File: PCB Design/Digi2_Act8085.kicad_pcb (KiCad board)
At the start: 2 copper layers, 27 parts, among them U1 8085A, U10 8255, U2 Barrel_Jack, U3 L7805, U4 2764, U5 CY6264, U6 74LS373, U7 74LS138, U8 8255, U9 8255, Y1 3MHz

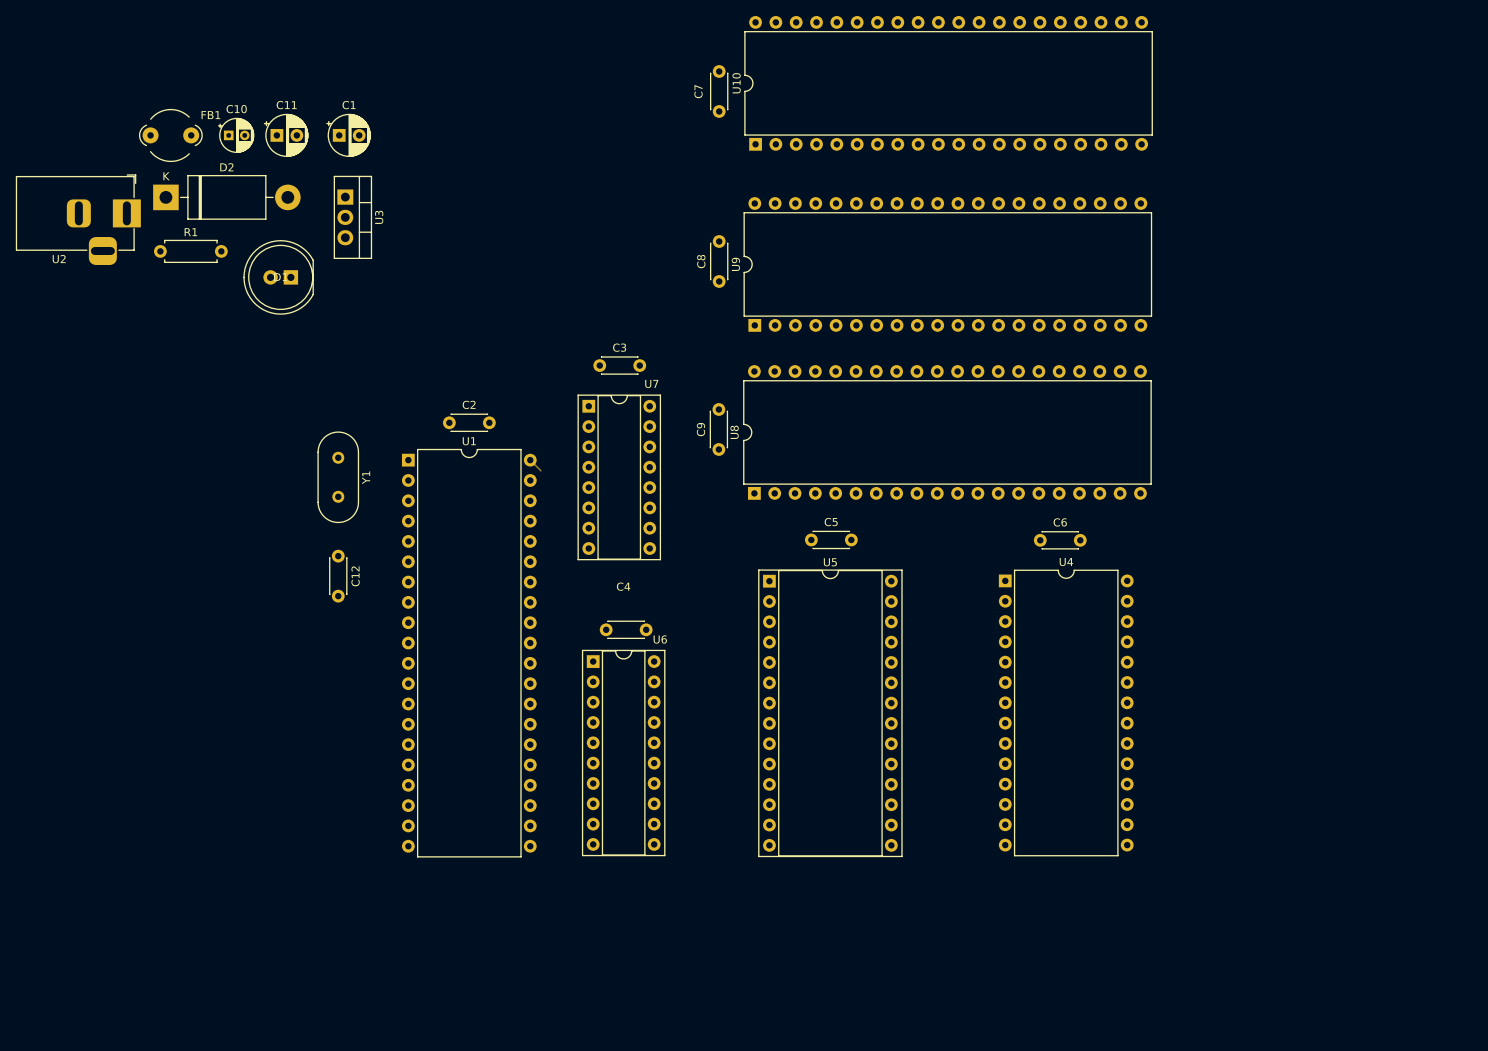
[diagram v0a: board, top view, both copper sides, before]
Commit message: Initial B
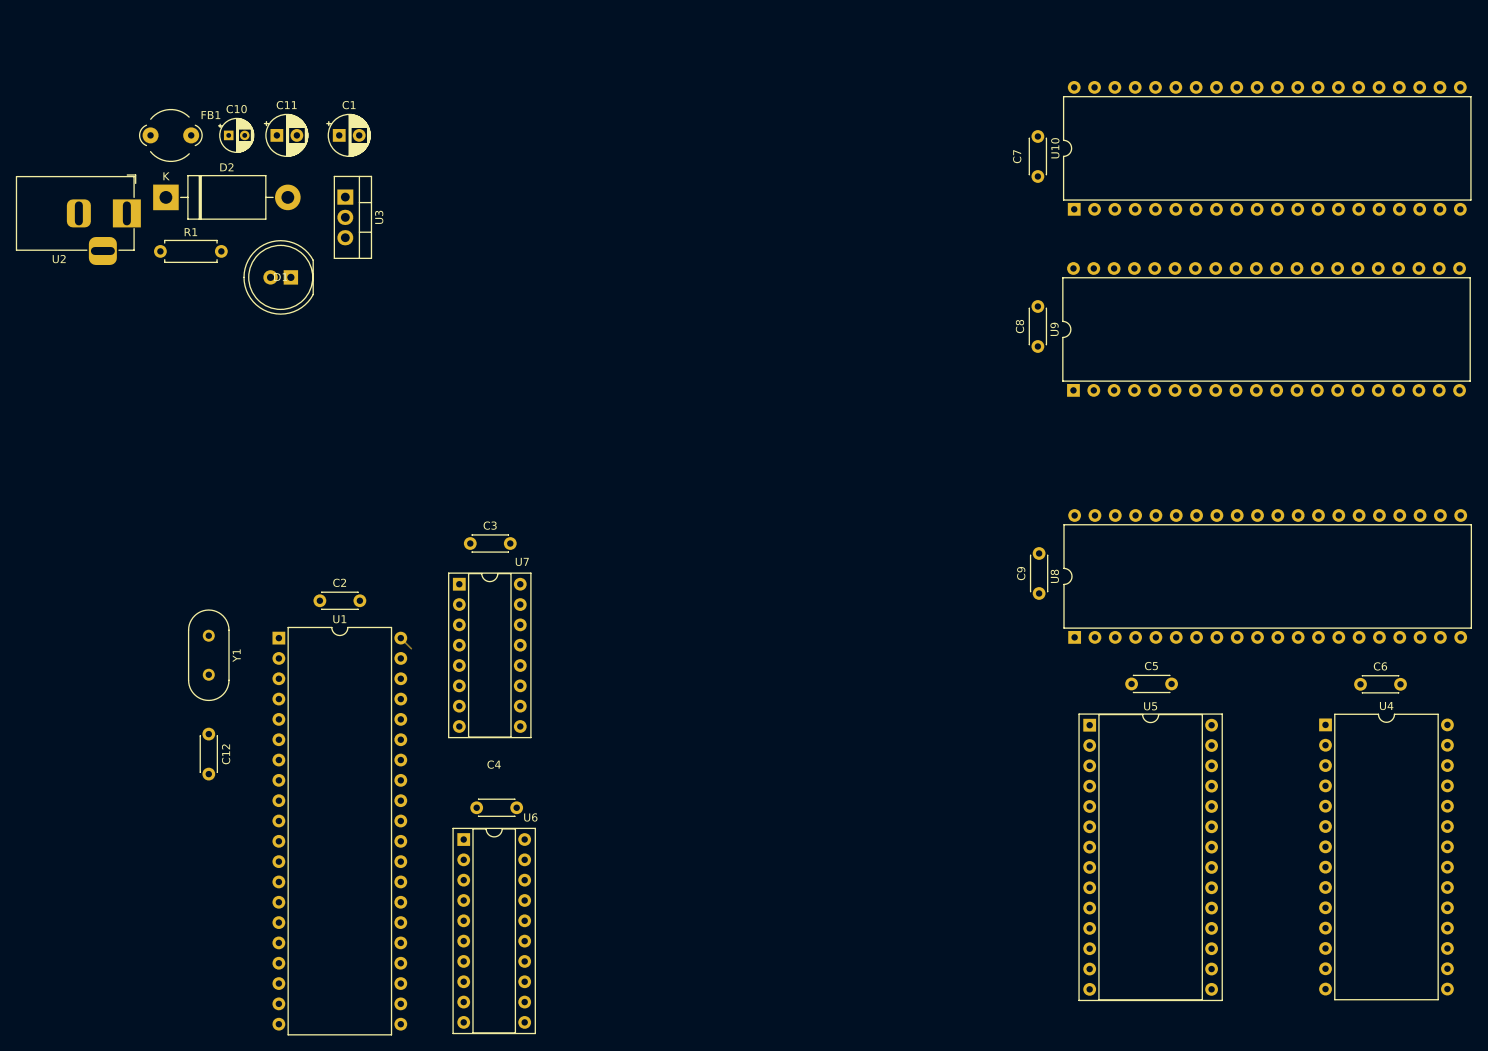
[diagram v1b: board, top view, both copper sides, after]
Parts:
- moved C5 43.9 mm to (168.1, 116.1)
- moved C6 43.9 mm to (196.7, 116.1)
- moved C9 43.9 mm to (156.5, 104.8)
- moved U4 43.9 mm to (192.3, 121.2)
- moved U5 43.9 mm to (162.8, 121.2)
- moved U8 43.9 mm to (161.0, 110.2)
- moved C7 40.7 mm to (156.4, 52.6)
- moved C8 40.7 mm to (156.4, 73.9)
- moved U10 40.7 mm to (160.9, 56.7)
- moved U9 40.7 mm to (160.8, 79.4)
- moved C2 27.5 mm to (66.6, 105.7)
- moved C3 27.5 mm to (85.4, 98.5)
- moved U1 27.5 mm to (61.5, 110.3)
- moved C12 27.5 mm to (52.7, 122.3)
- moved U7 27.5 mm to (84.1, 103.6)
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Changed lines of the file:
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@@
 	(footprint "Capacitor_THT:C_Disc_D4.3mm_W1.9mm_P5.00mm"
 		(layer "F.Cu")
-		(at 82.81 83.425)
+		(at 66.625 105.67)
 		(descr "C, Disc series, Radial, pin pitch=5.00mm, , diameter*width=4.3*1.9mm^2, Capacitor, http://www.vishay.com/docs/45233/krseries.pdf")
 		(tags "C Disc series Radial pin pitch 5.00mm  diameter 4.3mm width 1.9mm Capacitor")
@@
 	(footprint "Crystal:Crystal_HC49-U_Vertical"
 		(layer "F.Cu")
-		(at 68.925 87.795 -90)
+		(at 52.74 110.04 -90)
 		(descr "Crystal THT HC-49/U http://5hertz.com/pdfs/04404_D.pdf")
 		(tags "THT crystalHC-49/U")
@@
 	(footprint "Package_DIP:DIP-16_W7.62mm_Socket"
 		(layer "F.Cu")
-		(at 100.24 81.36)
+		(at 84.055 103.605)
 		(descr "16-lead though-hole mounted DIP package, row spacing 7.62 mm (300 mils), Socket")
 		(tags "THT DIP DIL PDIP 2.54mm 7.62mm 300mil Socket")
@@
 	(footprint "Package_DIP:DIP-20_W7.62mm_Socket"
 		(layer "F.Cu")
-		(at 100.79 113.27)
+		(at 84.605 135.515)
 		(descr "20-lead though-hole mounted DIP package, row spacing 7.62 mm (300 mils), Socket")
 		(tags "THT DIP DIL PDIP 2.54mm 7.62mm 300mil Socket")
 		(property "Reference" "U6"
-			(at 8.37 -2.72 360)
+			(at 8.37 -2.72 0)
 			(layer "F.SilkS")
 			(effects
@@
 		)
 		(property "Value" "74LS373"
-			(at 7.945 26.37 360)
+			(at 7.945 26.37 0)
 			(layer "F.Fab")
 			(effects
@@
 		)
 		(fp_text user "${REFERENCE}"
-			(at 7.945 12.61 360)
+			(at 7.945 12.61 0)
 			(layer "F.Fab")
 			(effects
@@
 	(footprint "Capacitor_THT:C_Disc_D4.3mm_W1.9mm_P5.00mm"
 		(layer "F.Cu")
-		(at 116.5 86.76 90)
+		(at 156.53 104.76 90)
 		(descr "C, Disc series, Radial, pin pitch=5.00mm, , diameter*width=4.3*1.9mm^2, Capacitor, http://www.vishay.com/docs/45233/krseries.pdf")
 		(tags "C Disc series Radial pin pitch 5.00mm  diameter 4.3mm width 1.9mm Capacitor")
 		(property "Reference" "C9"
-			(at 2.5 -2.2 270)
+			(at 2.5 -2.2 -90)
 			(layer "F.SilkS")
 			(effects
@@
 		)
 		(property "Value" "100nF"
-			(at 2.5 2.2 270)
+			(at 2.5 2.2 -90)
 			(layer "F.Fab")
 			(effects
@@
 		)
 		(fp_text user "${REFERENCE}"
-			(at 2.5 0 270)
+			(at 2.5 0 -90)
 			(layer "F.Fab")
 			(effects
@@
 	(footprint "Package_DIP:DIP-40_W15.24mm"
 		(layer "F.Cu")
-		(at 121.085 48.615 90)
+		(at 160.92 56.74 90)
 		(descr "40-lead though-hole mounted DIP package, row spacing 15.24 mm (600 mils)")
 		(tags "THT DIP DIL PDIP 2.54mm 15.24mm 600mil")
 		(property "Reference" "U10"
-			(at 7.62 -2.33 270)
+			(at 7.62 -2.33 -90)
 			(layer "F.SilkS")
 			(effects
@@
 		)
 		(property "Value" "8255"
-			(at 7.62 50.59 270)
+			(at 7.62 50.59 -90)
 			(layer "F.Fab")
 			(effects
@@
 		)
 		(fp_text user "${REFERENCE}"
-			(at 7.62 24.13 270)
+			(at 7.62 24.13 -90)
 			(layer "F.Fab")
 			(effects
@@
 	(footprint "Capacitor_THT:C_Disc_D4.3mm_W1.9mm_P5.00mm"
 		(layer "F.Cu")
-		(at 101.61 76.27)
+		(at 85.425 98.515)
 		(descr "C, Disc series, Radial, pin pitch=5.00mm, , diameter*width=4.3*1.9mm^2, Capacitor, http://www.vishay.com/docs/45233/krseries.pdf")
 		(tags "C Disc series Radial pin pitch 5.00mm  diameter 4.3mm width 1.9mm Capacitor")
@@
 	(footprint "Package_DIP:DIP-28_W15.24mm_Socket"
 		(layer "F.Cu")
-		(at 122.82 103.225)
+		(at 162.85 121.225)
 		(descr "28-lead though-hole mounted DIP package, row spacing 15.24 mm (600 mils), Socket")
 		(tags "THT DIP DIL PDIP 2.54mm 15.24mm 600mil Socket")
@@
 	(footprint "Package_DIP:DIP-28_W15.24mm"
 		(layer "F.Cu")
-		(at 152.3 103.19)
+		(at 192.33 121.19)
 		(descr "28-lead though-hole mounted DIP package, row spacing 15.24 mm (600 mils)")
 		(tags "THT DIP DIL PDIP 2.54mm 15.24mm 600mil")
@@
 	(footprint "Capacitor_THT:C_Disc_D4.3mm_W1.9mm_P5.00mm"
 		(layer "F.Cu")
-		(at 116.54 65.76 90)
+		(at 156.375 73.885 90)
 		(descr "C, Disc series, Radial, pin pitch=5.00mm, , diameter*width=4.3*1.9mm^2, Capacitor, http://www.vishay.com/docs/45233/krseries.pdf")
 		(tags "C Disc series Radial pin pitch 5.00mm  diameter 4.3mm width 1.9mm Capacitor")
 		(property "Reference" "C8"
-			(at 2.5 -2.2 270)
+			(at 2.5 -2.2 -90)
 			(layer "F.SilkS")
 			(effects
@@
 		)
 		(property "Value" "100nF"
-			(at 2.5 2.2 270)
+			(at 2.5 2.2 -90)
 			(layer "F.Fab")
 			(effects
@@
 		)
 		(fp_text user "${REFERENCE}"
-			(at 2.5 0 270)
+			(at 2.5 0 -90)
 			(layer "F.Fab")
 			(effects
@@
 	(footprint "Capacitor_THT:C_Disc_D4.3mm_W1.9mm_P5.00mm"
 		(layer "F.Cu")
-		(at 128.06 98.07)
+		(at 168.09 116.07)
 		(descr "C, Disc series, Radial, pin pitch=5.00mm, , diameter*width=4.3*1.9mm^2, Capacitor, http://www.vishay.com/docs/45233/krseries.pdf")
 		(tags "C Disc series Radial pin pitch 5.00mm  diameter 4.3mm width 1.9mm Capacitor")
@@
 	(footprint "Package_DIP:DIP-40_W15.24mm"
 		(layer "F.Cu")
-		(at 77.685 88.095)
+		(at 61.5 110.34)
 		(descr "40-lead though-hole mounted DIP package, row spacing 15.24 mm (600 mils)")
 		(tags "THT DIP DIL PDIP 2.54mm 15.24mm 600mil")
@@
 	(footprint "Package_DIP:DIP-40_W15.24mm"
 		(layer "F.Cu")
-		(at 120.94 92.25 90)
+		(at 160.97 110.25 90)
 		(descr "40-lead though-hole mounted DIP package, row spacing 15.24 mm (600 mils)")
 		(tags "THT DIP DIL PDIP 2.54mm 15.24mm 600mil")
 		(property "Reference" "U8"
-			(at 7.62 -2.44 270)
+			(at 7.62 -2.44 -90)
 			(layer "F.SilkS")
 			(effects
@@
 		)
 		(property "Value" "8255"
-			(at 7.62 50.59 270)
+			(at 7.62 50.59 -90)
 			(layer "F.Fab")
 			(effects
@@
 		)
 		(fp_text user "${REFERENCE}"
-			(at 7.62 24.13 270)
+			(at 7.62 24.13 -90)
 			(layer "F.Fab")
 			(effects
@@
 	(footprint "Capacitor_THT:C_Disc_D4.3mm_W1.9mm_P5.00mm"
 		(layer "F.Cu")
-		(at 68.925 100.092349 -90)
+		(at 52.74 122.337349 -90)
 		(descr "C, Disc series, Radial, pin pitch=5.00mm, , diameter*width=4.3*1.9mm^2, Capacitor, http://www.vishay.com/docs/45233/krseries.pdf")
 		(tags "C Disc series Radial pin pitch 5.00mm  diameter 4.3mm width 1.9mm Capacitor")
@@
 	(footprint "Package_DIP:DIP-40_W15.24mm"
 		(layer "F.Cu")
-		(at 120.99 71.25 90)
+		(at 160.825 79.375 90)
 		(descr "40-lead though-hole mounted DIP package, row spacing 15.24 mm (600 mils)")
 		(tags "THT DIP DIL PDIP 2.54mm 15.24mm 600mil")
 		(property "Reference" "U9"
-			(at 7.62 -2.33 270)
+			(at 7.62 -2.33 -90)
 			(layer "F.SilkS")
 			(effects
@@
 		)
 		(property "Value" "8255"
-			(at 7.62 50.59 270)
+			(at 7.62 50.59 -90)
 			(layer "F.Fab")
 			(effects
@@
 		)
 		(fp_text user "${REFERENCE}"
-			(at 7.62 24.13 270)
+			(at 7.62 24.13 -90)
 			(layer "F.Fab")
 			(effects
@@
 	(footprint "Capacitor_THT:C_Disc_D4.3mm_W1.9mm_P5.00mm"
 		(layer "F.Cu")
-		(at 102.41 109.3)
+		(at 86.225 131.545)
 		(descr "C, Disc series, Radial, pin pitch=5.00mm, , diameter*width=4.3*1.9mm^2, Capacitor, http://www.vishay.com/docs/45233/krseries.pdf")
 		(tags "C Disc series Radial pin pitch 5.00mm  diameter 4.3mm width 1.9mm Capacitor")
 		(property "Reference" "C4"
-			(at 2.18 -5.355 360)
+			(at 2.18 -5.355 0)
 			(layer "F.SilkS")
 			(effects
@@
 		)
 		(property "Value" "100nF"
-			(at 2.5 2.2 360)
+			(at 2.5 2.2 0)
 			(layer "F.Fab")
 			(effects
@@
 		)
 		(fp_text user "${REFERENCE}"
-			(at 2.5 0 360)
+			(at 2.5 0 0)
 			(layer "F.Fab")
 			(effects
@@
 	(footprint "Capacitor_THT:C_Disc_D4.3mm_W1.9mm_P5.00mm"
 		(layer "F.Cu")
-		(at 156.675 98.115)
+		(at 196.705 116.115)
 		(descr "C, Disc series, Radial, pin pitch=5.00mm, , diameter*width=4.3*1.9mm^2, Capacitor, http://www.vishay.com/docs/45233/krseries.pdf")
 		(tags "C Disc series Radial pin pitch 5.00mm  diameter 4.3mm width 1.9mm Capacitor")
@@
 	(footprint "Capacitor_THT:C_Disc_D4.3mm_W1.9mm_P5.00mm"
 		(layer "F.Cu")
-		(at 116.54 44.51 90)
+		(at 156.375 52.635 90)
 		(descr "C, Disc series, Radial, pin pitch=5.00mm, , diameter*width=4.3*1.9mm^2, Capacitor, http://www.vishay.com/docs/45233/krseries.pdf")
 		(tags "C Disc series Radial pin pitch 5.00mm  diameter 4.3mm width 1.9mm Capacitor")
 		(property "Reference" "C7"
-			(at 2.5 -2.55 270)
+			(at 2.5 -2.55 -90)
 			(layer "F.SilkS")
 			(effects
@@
 		)
 		(property "Value" "100nF"
-			(at 2.5 2.2 270)
+			(at 2.5 2.2 -90)
 			(layer "F.Fab")
 			(effects
@@
 		)
 		(fp_text user "${REFERENCE}"
-			(at 2.5 0 270)
+			(at 2.5 0 -90)
 			(layer "F.Fab")
 			(effects
@@
 	)
 	(segment
-		(start 92.925 88.095)
-		(end 94.255 89.425)
+		(start 76.74 110.34)
+		(end 78.07 111.67)
 		(width 0.2)
 		(layer "F.Cu")
